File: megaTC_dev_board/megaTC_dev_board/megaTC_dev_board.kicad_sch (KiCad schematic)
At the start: 35 parts, among them J1 Conn_01x08_Pin, J2 Conn_01x08_Pin, J3 Conn_01x08_Pin, U1 LTC2984CLX-PBF, U2 TPD4E1B06DCKR, U3 TPD4E1B06DCKR, U4 TPD4E1B06DCKR, U5 TPD4E1B06DCKR, U6 TPD4E1B06DCKR

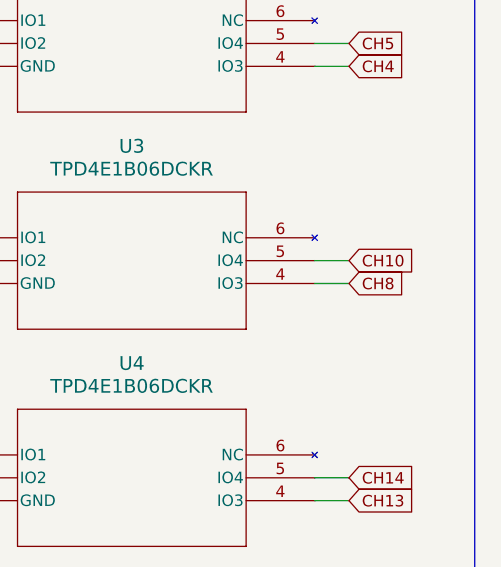
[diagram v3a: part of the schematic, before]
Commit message: routing wrap
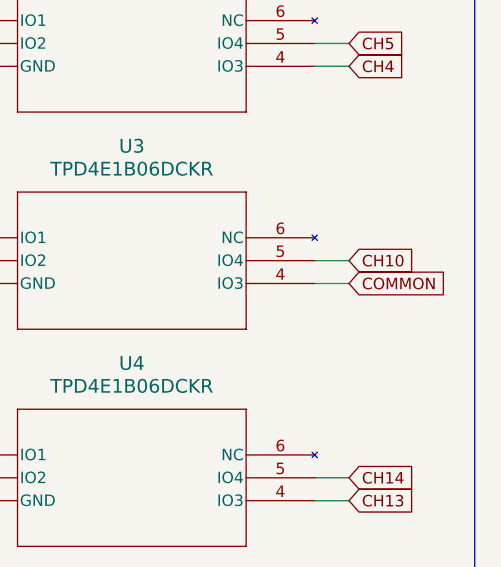
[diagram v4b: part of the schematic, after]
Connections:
- net CH8: no longer U3.4 (IO3)
- net COMMON: now also U3.4 (IO3)
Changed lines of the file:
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@@
 	(global_label "COMMON"
 		(shape input)
+		(at 351.79 87.63 0)
+		(fields_autoplaced yes)
+		(effects
+			(font
+				(size 1.27 1.27)
+			)
+			(justify left)
+		)
+		(property "Intersheetrefs" "${INTERSHEET_REFS}"
+			(at 362.9395 87.63 0)
+			(effects
+				(font
+					(size 1.27 1.27)
+				)
+				(justify left)
+				(hide yes)
+			)
+		)
+	)
+	(global_label "COMMON"
+		(shape input)
 		(at 154.94 186.69 0)
 		(fields_autoplaced yes)
@@
 				(hide yes)
 			)
-		)
-	)
-	(global_label "CH8"
-		(shape input)
-		(at 351.79 87.63 0)
-		(fields_autoplaced yes)
-		(effects
-			(font
-				(size 1.27 1.27)
-			)
-			(justify left)
-		)
-		(property "Intersheetrefs" "${INTERSHEET_REFS}"
-			(at 358.5852 87.63 0)
-			(effects
-				(font
-					(size 1.27 1.27)
-				)
-				(justify left)
-				(hide yes)
-			)

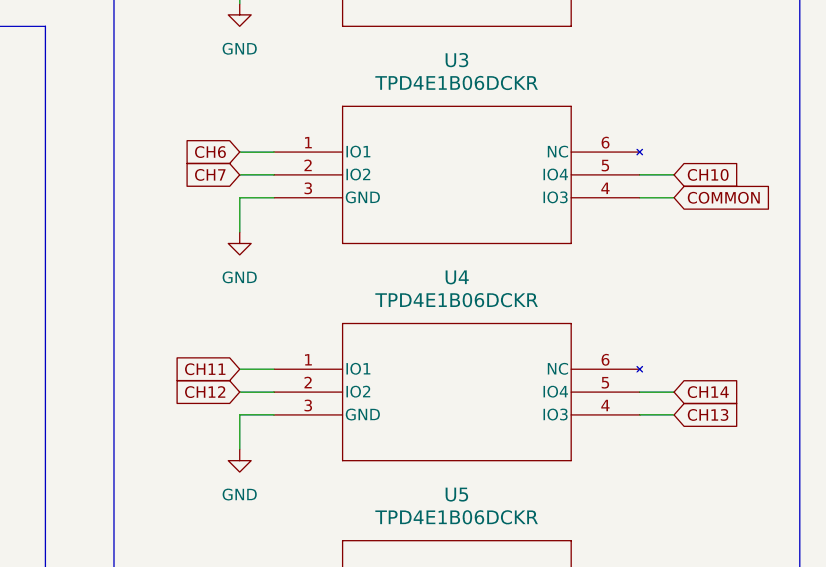
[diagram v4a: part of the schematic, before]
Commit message: routing progress
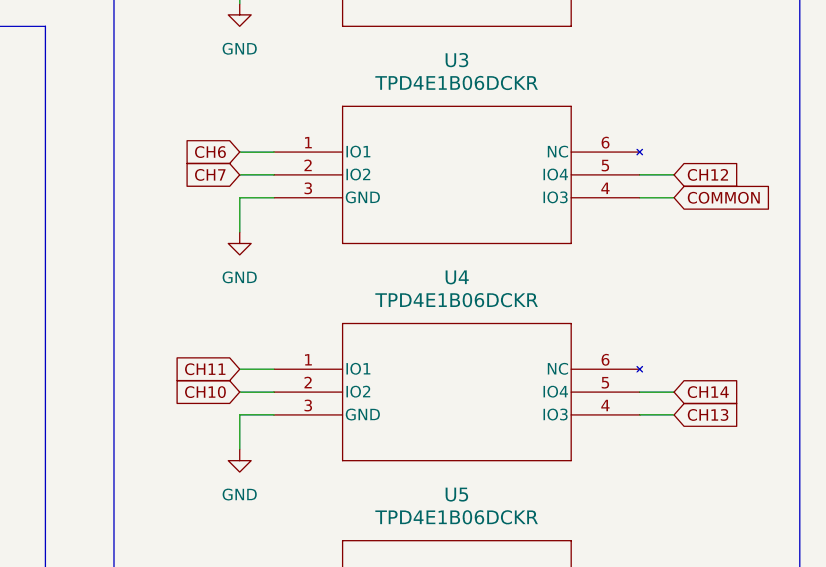
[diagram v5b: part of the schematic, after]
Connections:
- net CH10: now also U4.2 (IO2); no longer U3.5 (IO4)
- net CH12: now also U3.5 (IO4); no longer U4.2 (IO2)
